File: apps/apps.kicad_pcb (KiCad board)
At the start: 2 copper layers, 25 x 25 mm, 14 parts, among them J1 Conn_OUTPUT, Q1 SS9013, U1 XTR117

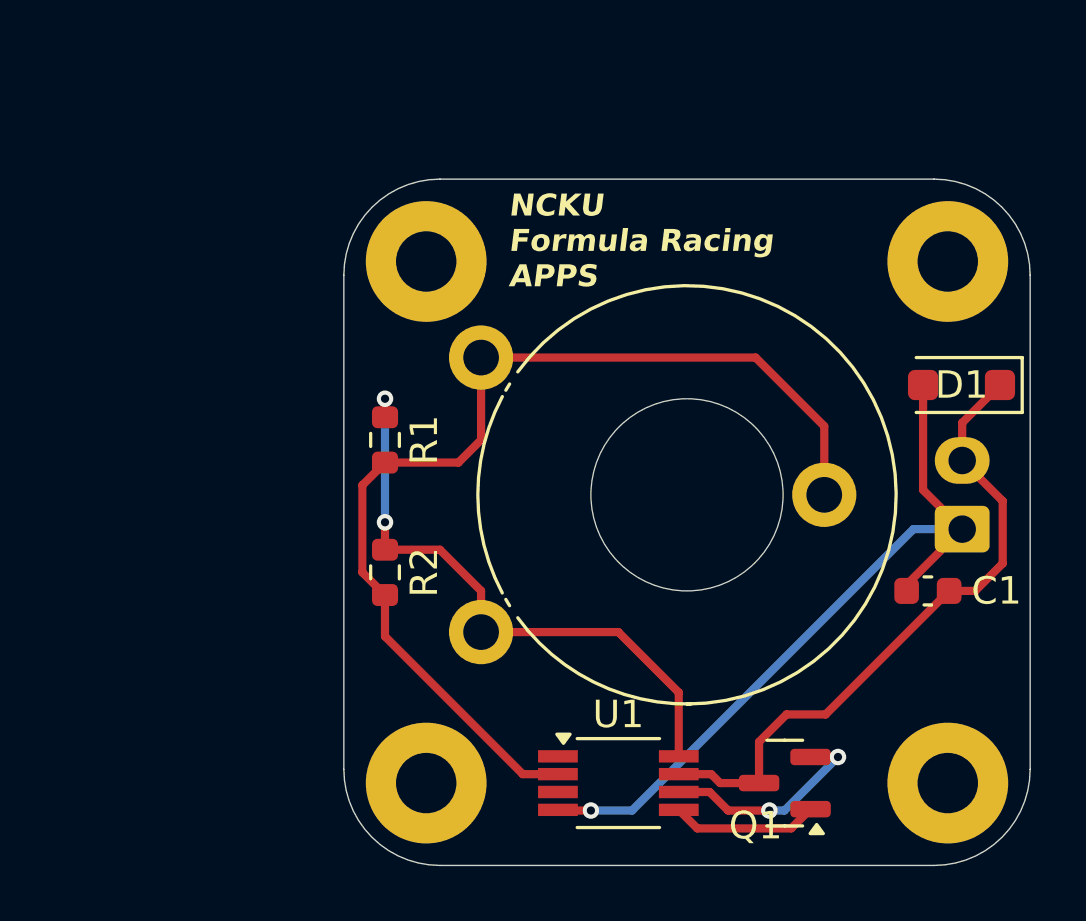
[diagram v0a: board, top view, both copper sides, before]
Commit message: feat: implement apps pcb
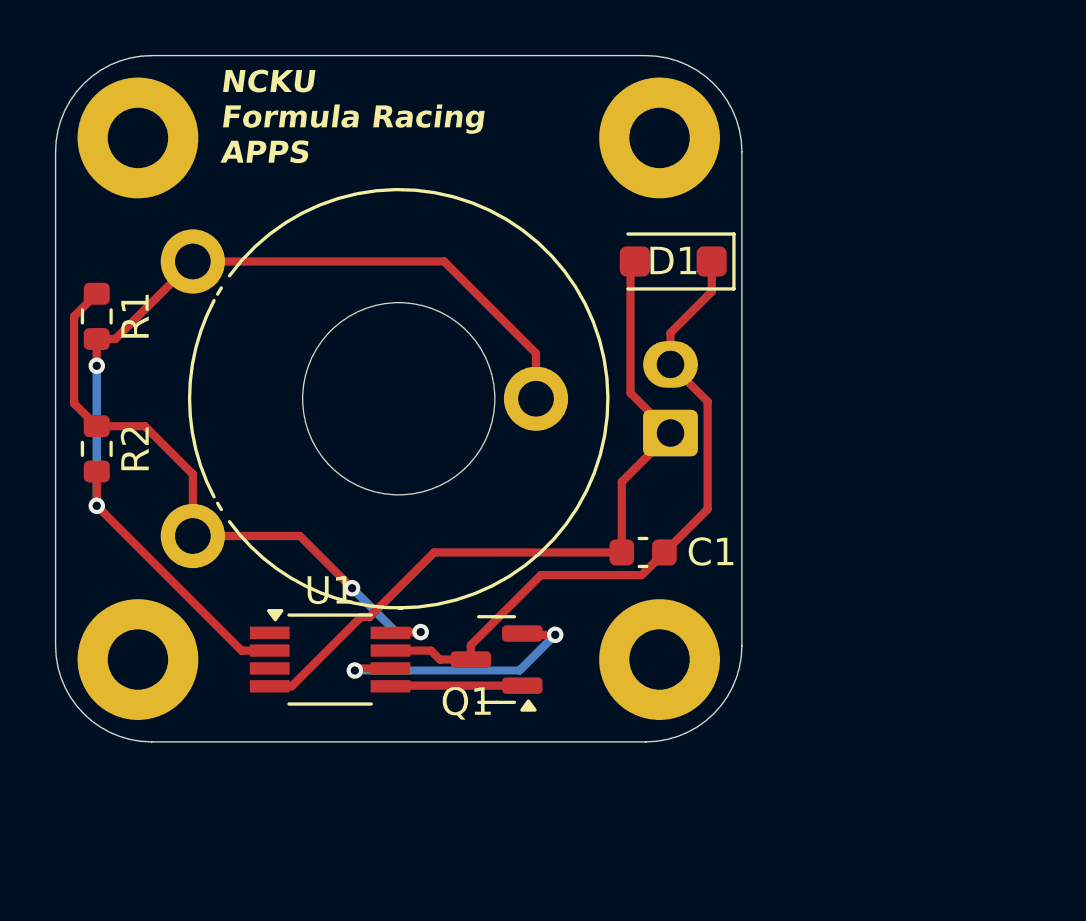
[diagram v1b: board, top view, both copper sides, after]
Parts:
- moved D1 11.4 mm to (101.0, 50.5)
- moved G*** 11.4 mm to (91.0, 45.0)
- moved G*** 11.4 mm to (91.0, 49.0)
- moved H1 11.4 mm to (100.5, 46.0)
- moved H2 11.4 mm to (100.5, 65.0)
- moved H3 11.4 mm to (81.5, 65.0)
- moved H4 11.4 mm to (81.5, 46.0)
- moved Q1 11.4 mm to (94.6, 65.0)
- moved R1 11.4 mm to (80.0, 52.5)
- moved R2 11.4 mm to (80.0, 57.3)
- moved U1 11.4 mm to (88.5, 65.0)
- moved J1 11.2 mm to (100.9, 56.8)
- moved RV1 11.1 mm to (83.5, 60.5)
- moved C1 10.5 mm to (99.9, 61.1)
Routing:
- net Net-(Q1-B): track 7.89 -> 10.4 mm
- net Net-(U1-IIN): track 38.3 -> 36.0 mm, vias 0 -> 2
- net Net-(D1-A): track 27.9 -> 26.8 mm, vias 1 -> 0
- net VDC: track 23.8 -> 24.5 mm
- net Net-(U1-VREG): track 22.2 -> 22.8 mm
- net Net-(Q1-E): track 5.37 -> 4.81 mm
